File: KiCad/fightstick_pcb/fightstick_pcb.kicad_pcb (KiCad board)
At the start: 2 copper layers, 93 parts, among them J1 USB_B_Micro, J2 Conn_01x02, J3 Conn_01x02, J4 Screw_Terminal_01x12, J5 Screw_Terminal_01x12, J6 Screw_Terminal_01x12, SW1 SW_Push, U1 SN74LVC1G14DBV, U10 SN74LVC1G14DBV, U11 SN74LVC1G14DBV, U12 SN74LVC1G14DBV, U13 SN74LVC1G14DBV, U14 SN74LVC1G14DBV, U15 SN74LVC1G14DBV, U2 SN74LVC1G14DBV, U3 NCP1117-3.3_SOT223, U4 W25Q128JVS, U5 SN74LVC1G14DBV, U6 SN74LVC1G14DBV, U7 SN74LVC1G14DBV, U8 SN74LVC1G14DBV, U9 RP2040, Y1 ABM8-272-T3

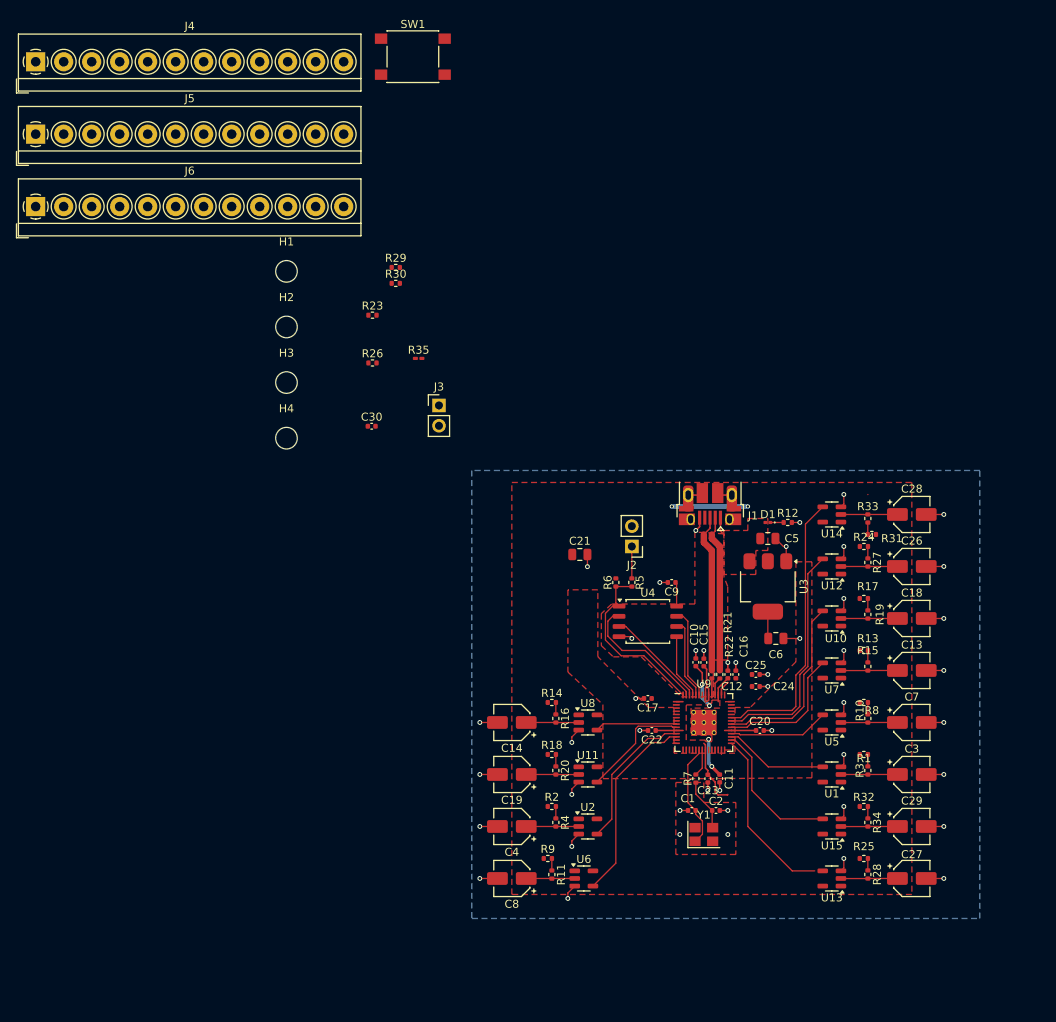
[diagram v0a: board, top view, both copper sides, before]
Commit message: PCB Fightstick V1
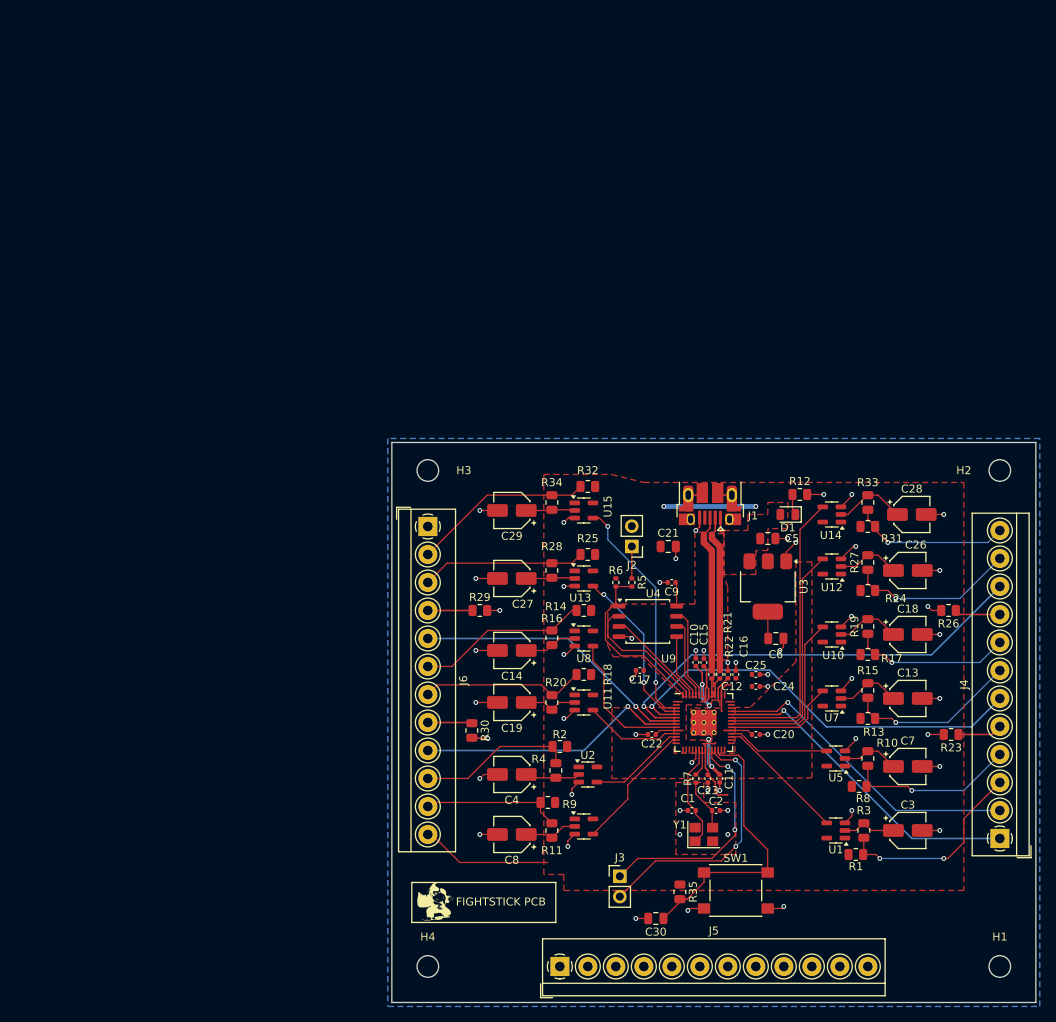
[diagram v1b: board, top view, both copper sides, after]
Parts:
- added G***: LOGO, LOGO, F.Cu at (66.5, 122.5)
- added REF**: KiCad-Logo2_5mm_SilkScreen, Symbol:KiCad-Logo2_5mm_SilkScreen, B.Cu at (72.0, 122.5)
- added REF**: WEEE-Logo_4.2x6mm_SilkScreen, Symbol:WEEE-Logo_4.2x6mm_SilkScreen, B.Cu at (74.0, 130.0)
- C30: footprint Capacitor_SMD:C_0402_1005Metric -> Capacitor_SMD:C_0805_2012Metric
- D1: footprint LED_SMD:LED_0201_0603Metric -> LED_SMD:LED_0805_2012Metric
- R1, R10, R11, R12, R13, R14, R15, R16, R17, R18, R19, R2, R20, R23, R24, R25, R26, R27, R28, R29, R3, R30, R31, R32, R33, R34, R4, R8, R9: footprint Resistor_SMD:R_0402_1005Metric -> Resistor_SMD:R_0805_2012Metric
- R35: footprint Resistor_SMD:R_0201_0603Metric_Pad0.64x0.40mm_HandSolder -> Resistor_SMD:R_0805_2012Metric
- moved J4 154.8 mm to (137.0, 114.5), turned to 90 degrees
- moved H1 124.5 mm to (137.0, 130.5)
- moved J5 123.0 mm to (82.0, 130.5)
- moved SW1 111.8 mm to (104.0, 121.0)
- moved H2 91.0 mm to (137.0, 68.5)
- moved R23 89.3 mm to (130.9, 101.5), turned to 180 degrees
- moved R26 78.4 mm to (130.6, 86.0), turned to 180 degrees
- moved R35 74.3 mm to (97.0, 121.2), turned to -90 degrees
- moved C30 71.0 mm to (94.0, 124.5), turned to 180 degrees
- moved H4 68.4 mm to (65.5, 130.5)
- moved C29 63.7 mm to (76.0, 73.5), turned to 180 degrees
- moved J6 63.3 mm to (65.5, 75.5), turned to -90 degrees
- moved J3 63.0 mm to (89.5, 119.2)
- moved C27 62.5 mm to (76.0, 82.0), turned to 180 degrees
- moved R30 56.7 mm to (71.0, 101.0), turned to -90 degrees
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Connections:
- J4 pad 1: /SW_1 -> /SIG_STICK_0
- J4 pad 10: /SW_RT -> /LED_P1+
- J4 pad 2: /SW_0 -> /SIG_STICK_1
- J4 pad 3: /SW_SELECT -> /SW_Y
- J4 pad 4: /SW_START -> /SW_X
- J4 pad 5: /SW_LB -> /LED_P0-
- J4 pad 6: /SW_RB -> /LED_P0+
- J4 pad 7: /SW_Y -> /SW_LT
- J4 pad 8: /SW_X -> /SW_RT
- J4 pad 9: /SW_LT -> /LED_P1-
- J6 pad 10: /LED_P0- -> /SW_1
- J6 pad 11: /LED_P0+ -> /SW_0
- J6 pad 2: /SIG_STICK_1 -> /SW_RB
- J6 pad 3: /SIG_STICK_0 -> /SW_LB
- J6 pad 4: /LED_P3- -> /LED_P2-
- J6 pad 5: /LED_P3+ -> /LED_P2+
- J6 pad 6: /LED_P2- -> /SW_SELECT
- J6 pad 7: /LED_P2+ -> /SW_START
- J6 pad 8: /LED_P1- -> /LED_P3-
- J6 pad 9: /LED_P1+ -> /LED_P3+
- U9 pad 11: /SIG_1 -> /SIG_START
- U9 pad 12: /SIG_0 -> /SIG_1
- U9 pad 13: unconnected-(U9-GPIO10-Pad13) -> /SIG_0
- U9 pad 2: /LED_P0+ -> unconnected-(U9-GPIO0-Pad2)
- U9 pad 29: /SIG_LB -> unconnected-(U9-GPIO18-Pad29)
- U9 pad 3: /LED_P1+ -> /SIG_RB
- U9 pad 30: /SIG_RB -> unconnected-(U9-GPIO19-Pad30)
- U9 pad 4: /LED_P2+ -> /SIG_LB
- U9 pad 5: /LED_P3+ -> /LED_P0+
- U9 pad 6: unconnected-(U9-GPIO4-Pad6) -> /LED_P1+
- U9 pad 7: unconnected-(U9-GPIO5-Pad7) -> /LED_P2+
- U9 pad 8: /SIG_SELECT -> /LED_P3+
- U9 pad 9: /SIG_START -> /SIG_SELECT
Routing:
- net /LED_P1+: track 0.00 -> 55.6 mm, vias 0 -> 1
- net /LED_P0+: track 0.00 -> 53.3 mm, vias 0 -> 1
- net /SIG_STICK_0: track 0.00 -> 40.4 mm, vias 0 -> 1
- net /SIG_STICK_1: track 0.00 -> 39.6 mm, vias 0 -> 1
- net /RUN: track 0.00 -> 35.6 mm
- net /LED_P2+: track 0.00 -> 35.3 mm, vias 0 -> 1
- net /LED_P3+: track 0.00 -> 34.3 mm, vias 0 -> 1
- net Net-(J3-Pin_2): track 0.00 -> 32.4 mm, vias 0 -> 2
- net Net-(J3-Pin_1): track 0.00 -> 29.0 mm, vias 0 -> 2
- net /SW_Y: track 1.49 -> 25.1 mm, vias 0 -> 2
- net +3V3: track 42.2 -> 64.9 mm
- net /SW_RB: track 1.49 -> 22.6 mm
- net GND: track 77.2 -> 98.2 mm, vias 46 -> 55
- net /SW_B: track 1.50 -> 21.6 mm, vias 0 -> 1
- net /SW_SELECT: track 1.49 -> 21.5 mm
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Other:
- board outline added: 80.5 x 70 mm
- board text added: "FIGHTSTICK PCB"
